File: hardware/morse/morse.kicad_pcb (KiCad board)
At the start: 2 copper layers, 85 x 54 mm, 25 parts, among them J1 Tag-Connect 6P Connector, Q1 SSM3J36FS, U1 ATtiny1617-M

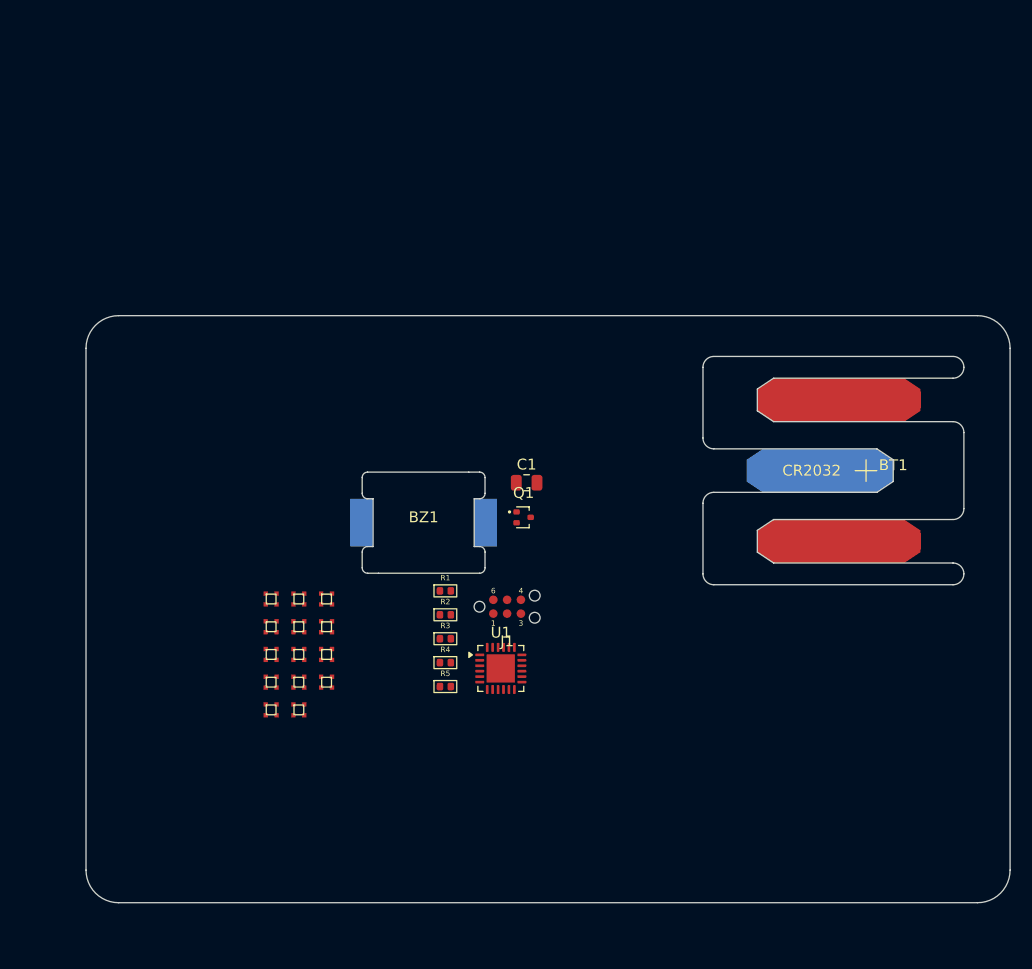
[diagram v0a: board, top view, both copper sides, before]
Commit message: Schematic progress
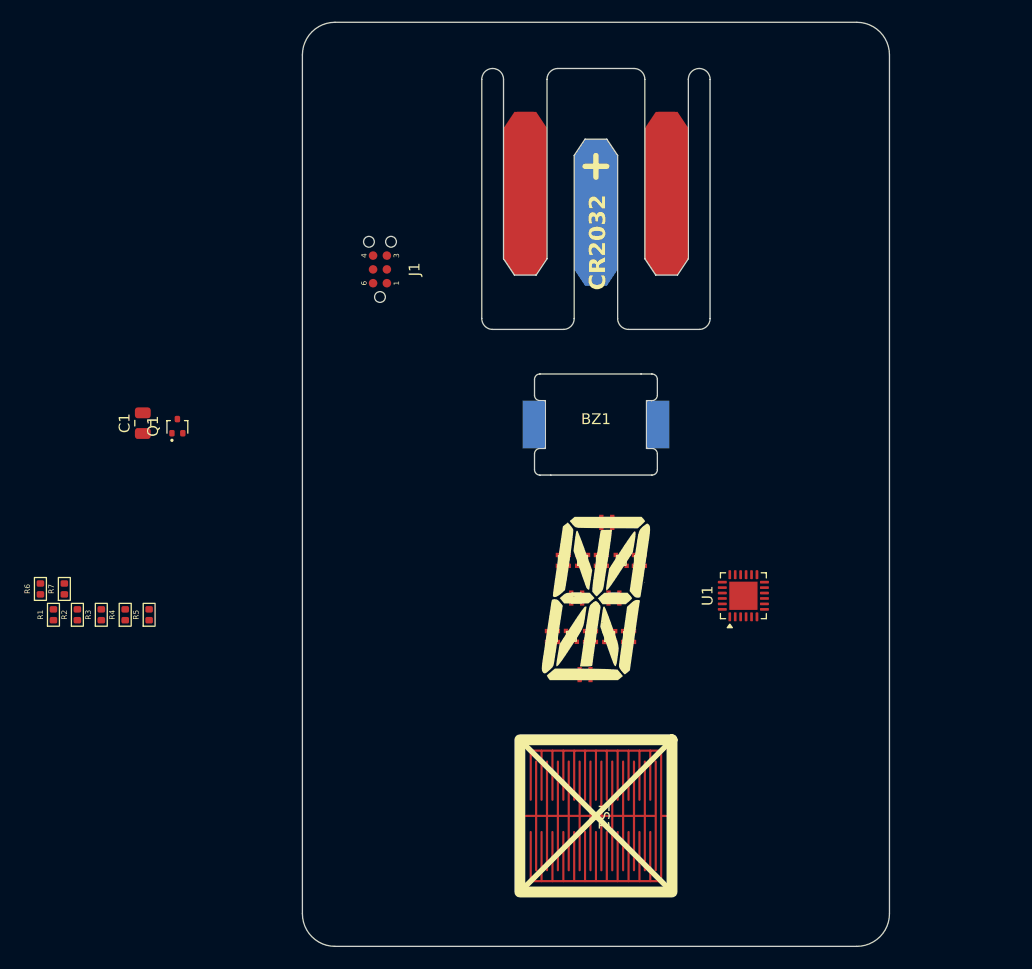
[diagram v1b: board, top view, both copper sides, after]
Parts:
- added G***: LOGO, libraries:14seg, F.Cu at (148.0, 97.5)
- added R6: 1k, libraries:Worthington_R_0402, F.Cu at (96.9, 96.6)
- added R7: 1k, libraries:Worthington_R_0402, F.Cu at (99.1, 96.6)
- added TS1: XY Touch Pad, libraries:TouchPad_12mm_XY, F.Cu at (148.0, 117.5)
- moved BT1 41.0 mm to (148.0, 55.2), turned to 90 degrees
- moved D5 36.6 mm to (152.0, 94.0), turned to 90 degrees
- moved R1 36.1 mm to (98.1, 99.0), turned to 90 degrees
- moved C1 35.7 mm to (106.3, 81.4), turned to 90 degrees
- moved R2 33.8 mm to (100.3, 99.0), turned to 90 degrees
- moved J1 33.2 mm to (128.1, 67.2), turned to 90 degrees
- moved Q1 32.9 mm to (109.5, 81.6), turned to 90 degrees
- moved R3 31.7 mm to (102.5, 99.0), turned to 90 degrees
- moved D1 31.7 mm to (149.0, 90.5), turned to 90 degrees
- moved D3 31.6 mm to (148.5, 94.0), turned to 90 degrees
- moved D4 31.4 mm to (149.3, 101.0), turned to 90 degrees
- moved D9 30.6 mm to (151.0, 101.0), turned to 90 degrees
- moved R4 29.8 mm to (104.7, 99.0), turned to 90 degrees
- moved D14 29.3 mm to (150.3, 94.0), turned to 90 degrees
- moved R5 28.0 mm to (106.9, 99.0), turned to 90 degrees
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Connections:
- J1 pad 3: GND -> unconnected-(J1-Pin_3-Pad3)
- J1 pad 4: unconnected-(J1-Pin_4-Pad4) -> GND
- J1 pad 5: unconnected-(J1-Pin_5-Pad5) -> /UPDI
- J1 pad 6: /UPDI -> +3V0
- U1 pad 15: unconnected-(U1-PB1-Pad15) -> /TOUCHY_T
- U1 pad 16: Net-(LA1--) -> /TOUCHX_T
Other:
- board size 85 x 54 mm -> 54 x 85 mm
